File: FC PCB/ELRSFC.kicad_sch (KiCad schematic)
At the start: 30 parts, among them SW1 SWITCH, U1 STM32F411RET6, U2 AMS1117-5.0, U3 AMS1117-3.3, X1 25MHz

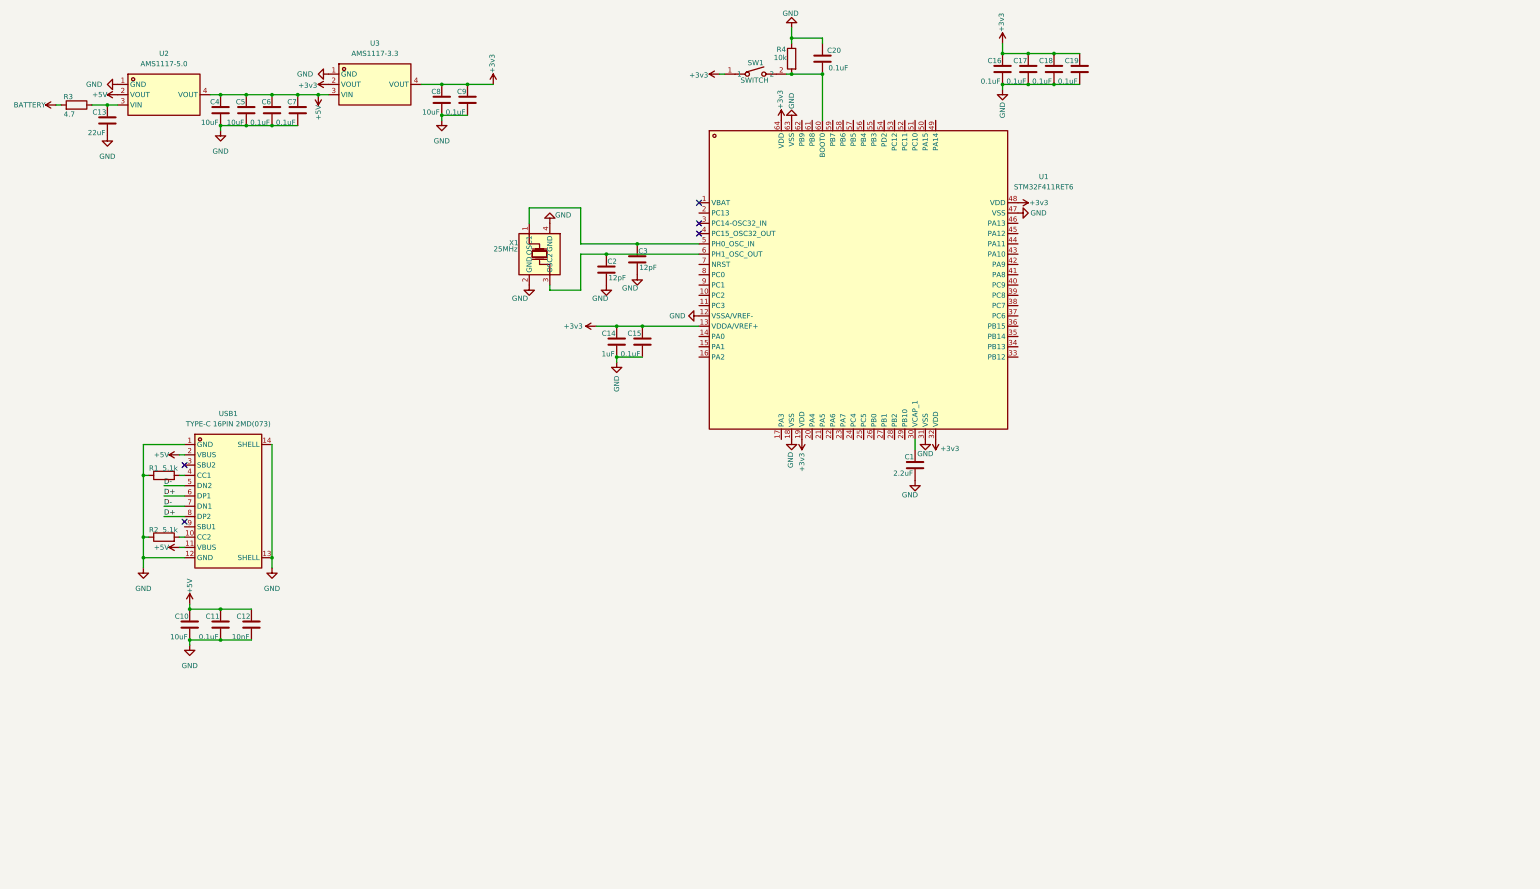
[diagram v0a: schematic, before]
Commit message: Fourth journal entry
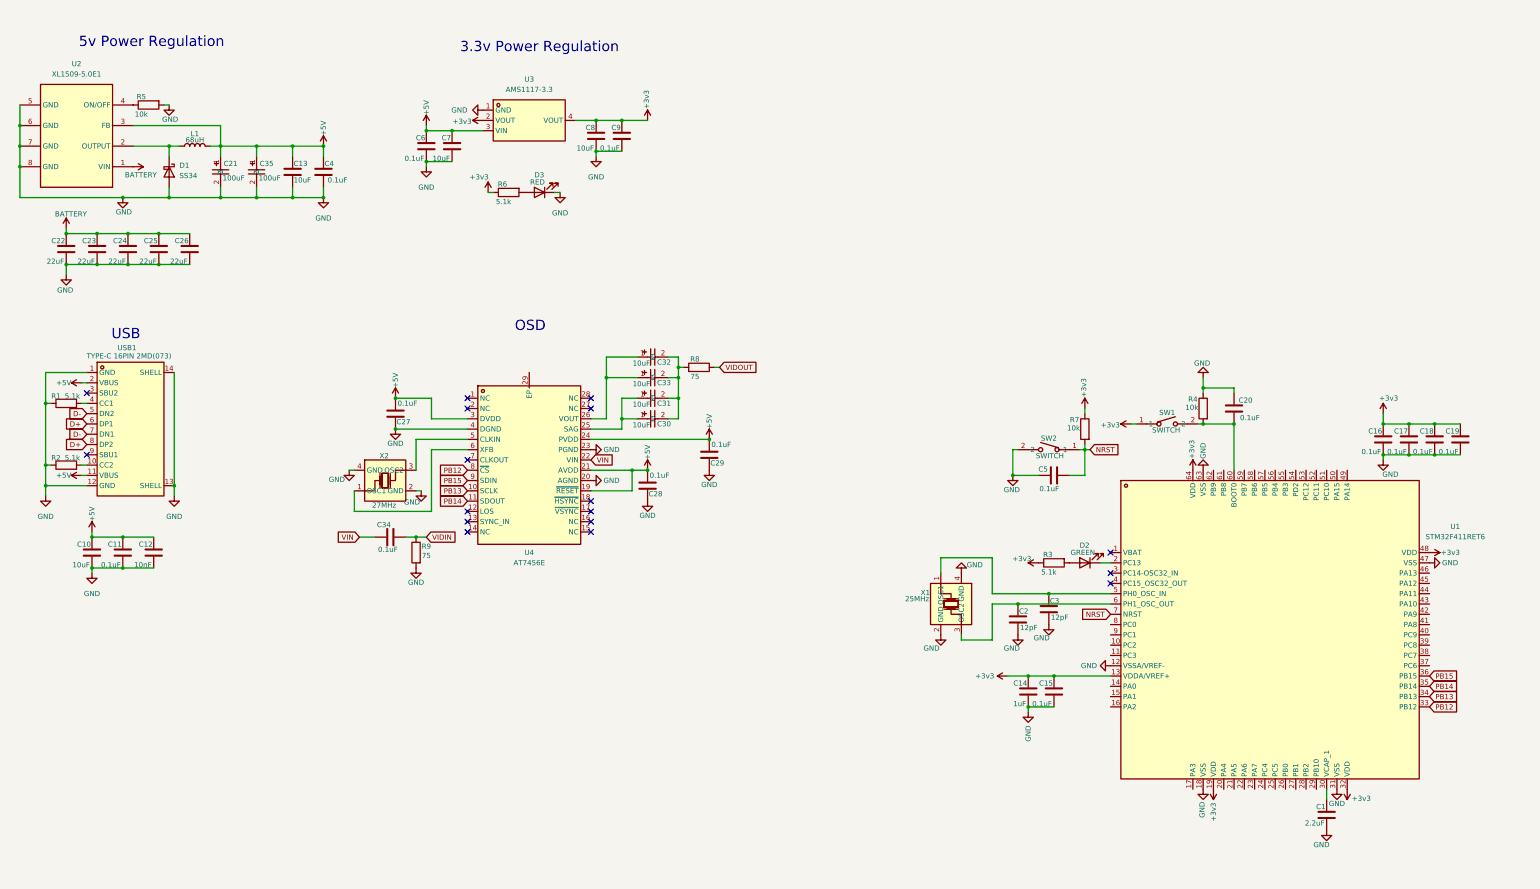
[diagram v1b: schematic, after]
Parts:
- removed U2: AMS1117-5.0, lcsc:SOT-223_L6.5-W3.5-P2.30-LS7.0-BR, symbol ELRSFC:AMS1117-5.0
- added C21, C35: 100uF, lcsc:CASE-B_3528, symbol ELRSFC:TAJB107K006RNJ
- added C22, C23, C24, C25, C26: 22uF, symbol Device:C
- added C27, C28, C29, C34: 0.1uF, symbol Device:C
- added C30, C31, C32, C33: 10uF, lcsc:CAP-SMD_L3.2-W1.6-RD-C7171, symbol ELRSFC:TAJA106K016RNJ
- added D1: SS34, Diode_SMD:D_SMA, symbol Diode:SS34
- added D2: GREEN, symbol Device:LED
- added D3: RED, symbol Device:LED
- added L1: 68uH, symbol Device:L
- added R5, R7: 10k, symbol Device:R
- added R6: 5.1k, symbol Device:R
- added R8, R9: 75, symbol Device:R
- added SW2: SWITCH, lcsc:SW-SMD_L3.9-W3.0-P4.45, symbol ELRSFC:TS-1088-AR02016
- added U2: XL1509-5.0E1, lcsc:SOIC-8_L5.0-W4.0-P1.27-LS6.0-BL, symbol ELRSFC:XL1509-5.0E1
- added U4: AT7456E, lcsc:TSSOP-28_L9.7-W4.4-P0.65-LS6.4-BL-EP-2, symbol ELRSFC:AT7456E
- added X2: 27MHz, lcsc:CRYSTAL-SMD_4P-L3.2-W2.5-BL, symbol ELRSFC:S3227000181040
- C13: value 22uF -> 10uF
- C4, C5: value 10uF -> 0.1uF
- C7: value 0.1uF -> 10uF
- R3: value 4.7 -> 5.1k
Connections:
- net +3v3: now also R3.1, R6.1, R7.1
- net +5V: now also C13.1, C21.1, C27.2, C28.2, C29.2, C35.1, L1.2, U2.3 (FB), U4.19 (~{RESET}), U4.21 (AVDD), U4.24 (PVDD), U4.3 (DVDD); no longer C5.1
- net BATTERY: now also C22.1, C23.1, C24.1, C25.1, C26.1, U2.1 (VIN); no longer R3.2
- net GND: now also C5.1, C21.2, C22.2, C23.2, C24.2, C25.2, C26.2, C27.1, C28.1, C29.1, C35.2, D1.2 (A), D3.1 (K), R5.2, R9.2, SW2.2, U2.5 (GND), U2.6 (GND), U2.7 (GND), U2.8 (GND), U4.20 (AGND), U4.23 (PGND), U4.4 (DGND), X2.2 (GND), X2.4 (GND); no longer C5.2
- net at U1.2 (PC13): now also D2.1 (K)
- net PB12: now reaches U1.33 (PB12)
- net PB12: now also U4.8 (~{CS})
- net PB13: now reaches U1.34 (PB13)
- net PB13: now also U4.10 (SCLK)
- net PB14: now reaches U1.35 (PB14)
- net PB14: now also U4.11 (SDOUT)
- net PB15: now reaches U1.36 (PB15)
- net PB15: now also U4.9 (SDIN)
- net NRST: now reaches U1.7 (NRST)
- net NRST: now also C5.2, R7.2, SW2.1
- new net: R5.1, U2.4 (ON/OFF)
- new net: C30.1, C31.1, U4.25 (SAG)
- new net: C32.1, C33.1, U4.26 (VOUT)
- new net: U4.5 (CLKIN), X2.3 (OSC2)
- new net: U4.6 (XFB), X2.1 (OSC1)
- new net: D1.1 (K), L1.1, U2.2 (OUTPUT)
- new net: C30.2, C31.2, C32.2, C33.2, R8.2
- new net: D3.2 (A), R6.2
- new net: D2.2 (A), R3.2
- new net VIDIN: C34.1, R9.1
- new net VIDOUT: R8.1
- new net VIN: C34.2, U4.22 (VIN)
- no-connect marks 5 -> 17
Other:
- note added: "3.3v Power Regulation"
- note added: "5v Power Regulation"
- note added: "OSD"
- note added: "USB"
- title: (none) -> Merlyn411
- moved on the sheet: C1, C10, C11, C12, C14, C15, C16, C17, C18, C19, C2, C20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

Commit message: Fifth journal entry
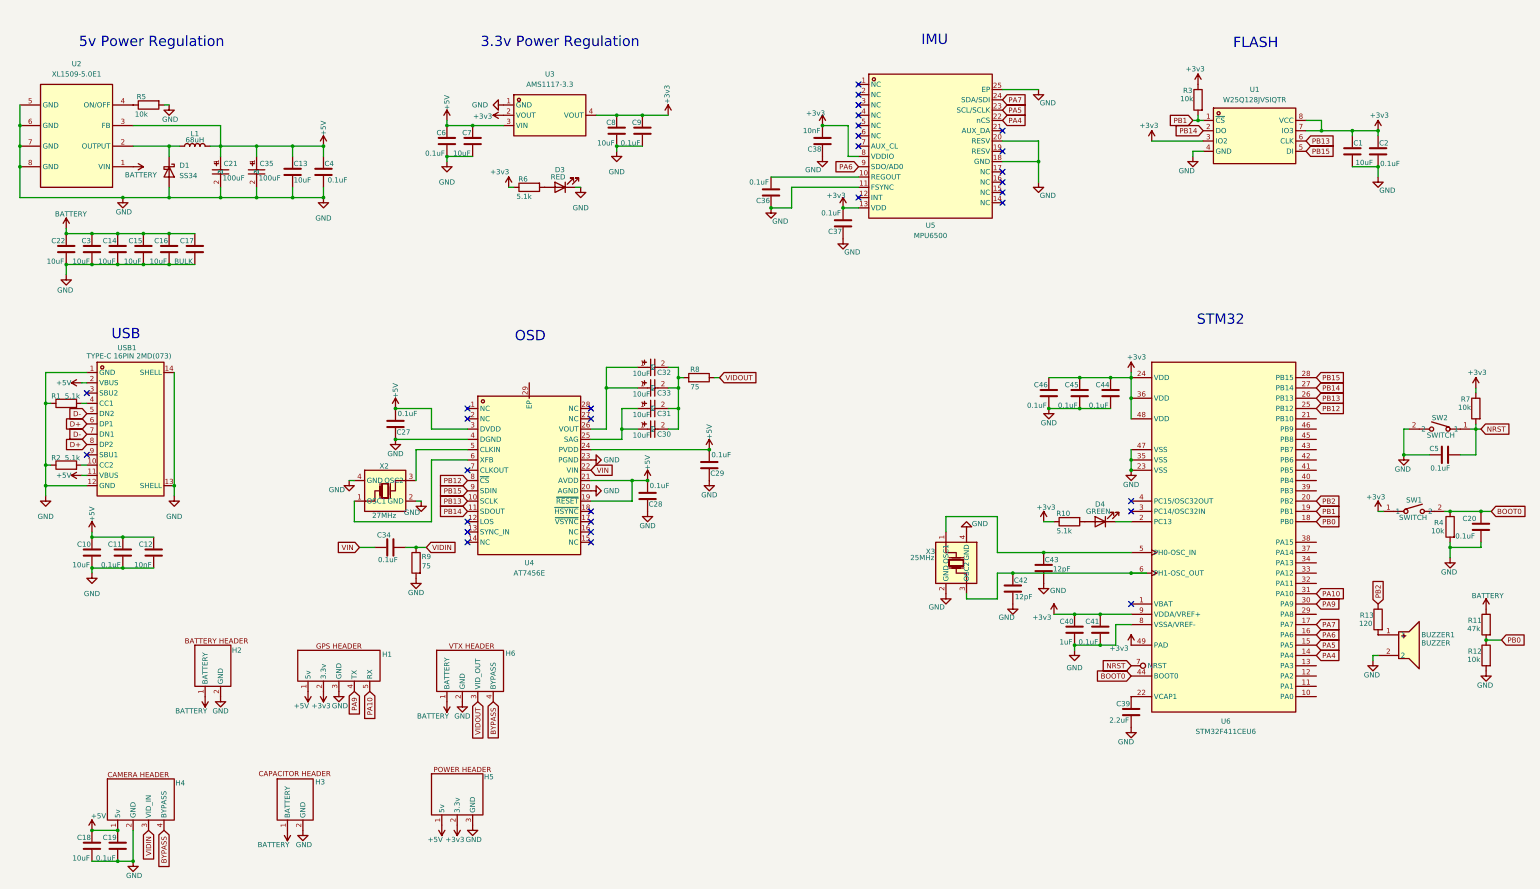
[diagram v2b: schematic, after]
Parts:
- removed C23, C24, C25, C26: 22uF, symbol Device:C
- removed D2: GREEN, symbol Device:LED
- removed U1: STM32F411RET6, lcsc:LQFP-64_L10.0-W10.0-P0.50-LS12.0-BL, symbol ELRSFC:STM32F411RET6
- removed X1: 25MHz, lcsc:CRYSTAL-SMD_4P-L3.2-W2.5-BL, symbol ELRSFC:X322525MOB4SI
- added BUZZER1: BUZZER, lcsc:BUZ-SMD_L9.6-W9.6-LS10.0-R, symbol ELRSFC:HND-9650B
- added C36, C37, C41, C44, C45, C46: 0.1uF, symbol Device:C
- added C38: 10nF, symbol Device:C
- added C39: 2.2uF, symbol Device:C
- added C40: 1uF, symbol Device:C
- added C42, C43: 12pF, symbol Device:C
- added D4: GREEN, symbol Device:LED
- added H1: ~, symbol ELRSFC:GPS
- added H2: ~, symbol ELRSFC:BATTERY
- added H3: ~, symbol ELRSFC:CAP
- added H4: ~, symbol ELRSFC:CAMERA
- added H5: ~, symbol ELRSFC:POWER
- added H6: ~, symbol ELRSFC:VTX
- added R10: 5.1k, symbol Device:R
- added R11: 47k, symbol Device:R
- added R12: 10k, symbol Device:R
- added R13: 120, symbol Device:R
- added U1: W25Q128JVSIQTR, lcsc:SOIC-8_L5.3-W5.3-P1.27-LS8.0-BL, symbol ELRSFC:W25Q128JVSIQTR
- added U5: MPU6500, lcsc:QFN-24_L3.0-W3.0-P0.40-BL-EP, symbol ELRSFC:MPU6500
- added U6: STM32F411CEU6, lcsc:UFQFPN-48_L7.0-W7.0-P0.50-BL-EP, symbol ELRSFC:STM32F411CEU6
- added X3: 25MHz, lcsc:CRYSTAL-SMD_4P-L3.2-W2.5-BL, symbol ELRSFC:X322525MOB4SI
- C1: value 2.2uF -> 10uF
- C14: value 1uF -> 10uF
- C15, C16, C18: value 0.1uF -> 10uF
- C17: value 0.1uF -> BULK
- C2: value 12pF -> 0.1uF
- C22: value 22uF -> 10uF
- C3: value 12pF -> 10uF
- R3: value 5.1k -> 10k
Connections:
- net +3v3: now also C1.1, C2.1, C37.2, C38.2, C40.1, C41.1, C44.1, C45.1, C46.1, H1.2 (3.3v), H5.2 (3.3v), R10.1, U1.3 (IO2), U1.7 (IO3), U1.8 (VCC), U5.13 (VDD), U5.8 (VDDIO), U6.24 (VDD), U6.36 (VDD), U6.48 (VDD), U6.49 (PAD), U6.9 (VDDA/VREF+); no longer C14.1, C15.1, C16.1, C17.1, C18.1, C19.1
- net +5V: now also C18.1, C19.1, H1.1 (5v), H4.1 (5v), H5.1 (5v)
- net BATTERY: now also C14.1, C15.1, C16.1, C17.1, C3.1, H2.1 (BATTERY), H3.1 (BATTERY), H6.1 (BATTERY), R11.1
- net GND: now also C20.2, R4.2, BUZZER1.2, C36.1, C37.1, C38.1, C39.2, C40.2, C41.2, C42.2, C43.2, C44.2, C45.2, C46.2, H1.3 (GND), H2.2 (GND), H3.2 (GND), H4.2 (GND), H5.3 (GND), H6.2 (GND), R12.2, U1.4 (GND), U5.11 (FSYNC), U5.18 (GND), U5.20 (RESV), U5.25 (EP), U6.23 (VSS), U6.35 (VSS), U6.47 (VSS), U6.8 (VSSA/VREF-), X3.2 (GND), X3.4 (GND); no longer C20.1, R4.1
- net NRST: now also U6.7 (NRST)
- net PB12: now also U6.25 (PB12)
- net PB13: now also U1.6 (CLK), U6.26 (PB13)
- net PB14: now also U1.2 (DO), U6.27 (PB14)
- net PB15: now also U1.5 (DI), U6.28 (PB15)
- net VIDIN: now also H4.3 (VID_IN)
- net VIDOUT: now also H6.3 (VID_OUT)
- net PB1: now reaches R3.2
- net PB1: now also U1.1 (~{CS}), U6.19 (PB1)
- new net: BUZZER1.1, R13.2
- new net: C43.1, U6.5 (PH0-OSC_IN), X3.1 (OSC1)
- new net: D4.2 (A), R10.2
- new net: C36.2, U5.10 (REGOUT)
- new net: D4.1 (K), U6.2 (PC13)
- new net: C39.1, U6.22 (VCAP1)
- new net: C42.1, U6.6 (PH1-OSC_OUT), X3.3 (OSC2)
- new net BOOT0: C20.1, R4.1, SW1.2, U6.44 (BOOT0)
- new net BYPASS: H4.4 (BYPASS), H6.4 (BYPASS)
- new net PA10: H1.5 (RX), U6.31 (PA10)
- new net PA4: U5.22 (nCS), U6.14 (PA4)
- new net PA5: U5.23 (SCL/SCLK), U6.15 (PA5)
- new net PA6: U5.9 (SDO/AD0), U6.16 (PA6)
- new net PA7: U5.24 (SDA/SDI), U6.17 (PA7)
- new net PA9: H1.4 (TX), U6.30 (PA9)
- new net PB0: R11.2, R12.1, U6.18 (PB0)
- new net PB2: R13.1, U6.20 (PB2)
- no-connect marks 17 -> 31
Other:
- note added: "FLASH"
- note added: "IMU"
- note added: "STM32"
- moved on the sheet: C20, C27, C28, C29, C30, C31, C32, C33, C34, C5, C6, C7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
